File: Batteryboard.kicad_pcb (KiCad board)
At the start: 4 copper layers, 75.8 x 76.2 mm, 143 parts, among them IC1 FAN4010IL6X_F113, IC2 FAN4010IL6X_F113, IC3 FAN4010IL6X_F113, J1 Conn_01x02_Male, J2 Conn_01x03_Male, J4 Conn_01x02_Male, J5 SC_19-20, Q1 SI7617DN-T1-GE3, Q2 SI7617DN-T1-GE3, Q3 SI7617DN-T1-GE3, Q4 SIS412DN-T1-GE3, Q5 SIS412DN-T1-GE3, Q6 SIS412DN-T1-GE3, Q7 SI7617DN-T1-GE3, Q8 SIS412DN-T1-GE3, U1 BQ24617RGET, U2 TPS65279DAPR, U3 BQ29200DRBT, U4 PIC18F25K50-I_SO, U5 MCP2515-xSO, U6 SN65HVD1050D

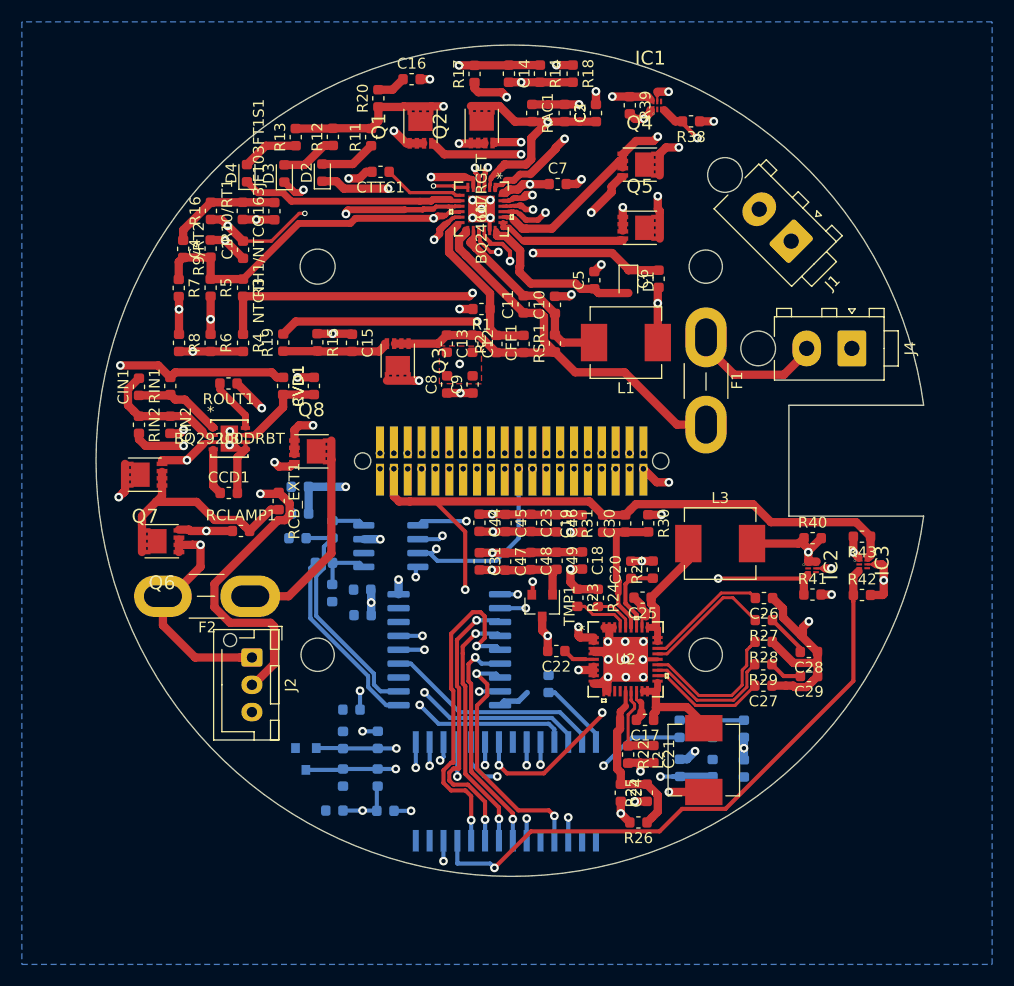
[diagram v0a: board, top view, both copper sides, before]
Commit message: complete overhaul of board, trying to make it a bit better
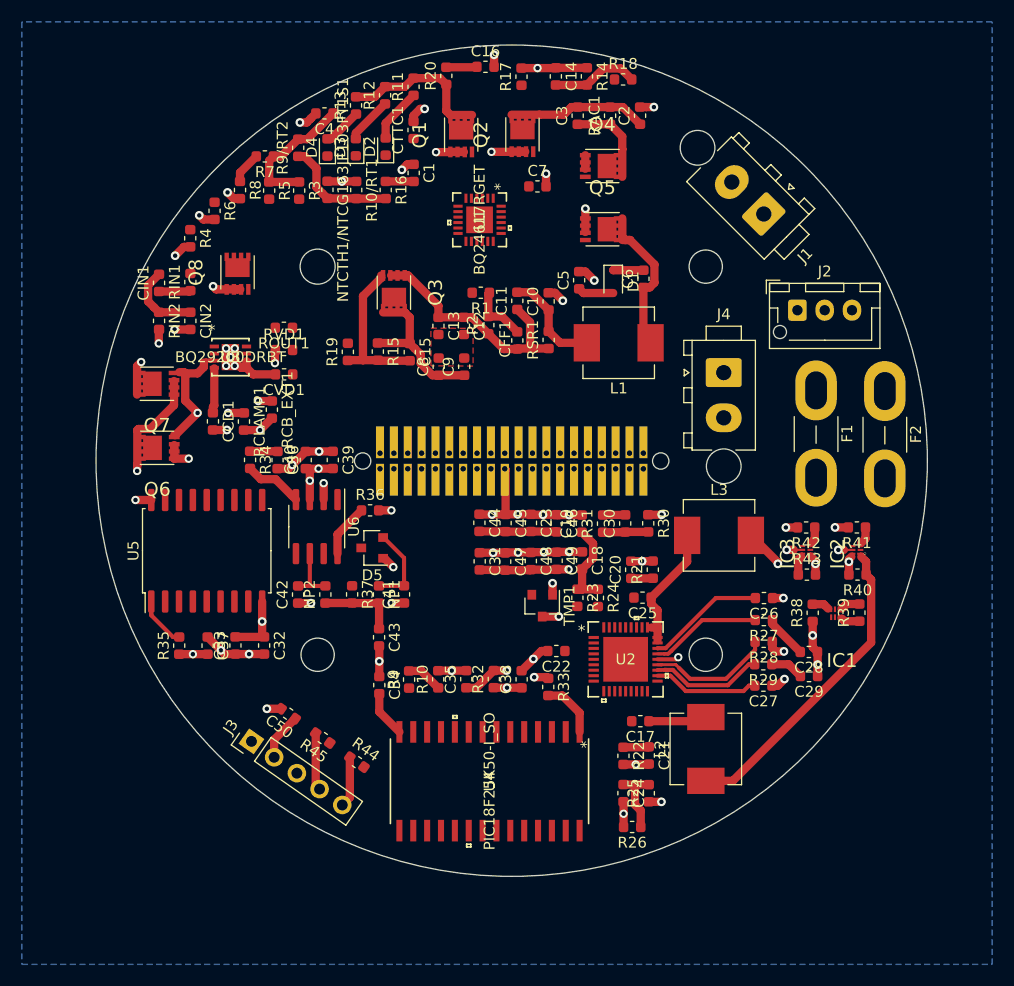
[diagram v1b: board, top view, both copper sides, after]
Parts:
- added C50: C, Capacitor_SMD:C_0603_1608Metric, F.Cu at (214.9, 86.2)
- added J3: Conn_01x05_Male, Connector_PinHeader_2.54mm:PinHeader_1x05_P2.54mm_Vertical, F.Cu at (211.5, 88.8)
- added R44: R_US, Resistor_SMD:R_0603_1608Metric, F.Cu at (221.2, 90.7)
- added R45: R_US, Resistor_SMD:R_0603_1608Metric, F.Cu at (218.1, 88.5)
- C32, C33, C34, C35, C36, C37, C38, C39, C40, C41, C42, C43, D5, NP1, NP2, R10, R32, R33, R34, R35, R36, R37, R9, U4, U5, U6: moved to F.Cu
- moved F2 61.1 mm to (269.6, 56.7), turned to 270 degrees
- moved J2 59.2 mm to (261.6, 49.3), turned to 0 degrees
- moved R39 51.0 mm to (267.2, 77.0), turned to 90 degrees
- moved IC1 49.3 mm to (265.0, 77.0), turned to 180 degrees
- moved R38 46.4 mm to (263.0, 77.0), turned to 90 degrees
- moved R10 26.4 mm to (228.7, 83.1)
- moved R9 26.1 mm to (226.0, 83.1), turned to 90 degrees
- moved U5 24.0 mm to (207.4, 71.3), turned to 90 degrees
- moved R32 23.4 mm to (233.7, 83.1)
- moved C35 23.0 mm to (231.2, 83.1), turned to 90 degrees
- moved C38 21.9 mm to (236.3, 83.1), turned to 90 degrees
- moved D5 20.3 mm to (222.6, 71.1), turned to 180 degrees
- moved R37 20.1 mm to (220.8, 75.3), turned to 270 degrees
- moved R36 18.3 mm to (222.4, 67.6), turned to 0 degrees
- moved Q8 17.7 mm to (210.3, 45.8), turned to 90 degrees
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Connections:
- C15 pad 1: 5V0 -> Q4D
- C23 pad 2: 5V0 -> Net-(C23-Pad2)
- C3 pad 1: 5V0 -> Q4D
- C31 pad 2: 5V0 -> Net-(C31-Pad2)
- C44 pad 2: 5V0 -> Net-(C23-Pad2)
- C45 pad 2: 5V0 -> Net-(C23-Pad2)
- C46 pad 2: 5V0 -> Net-(C23-Pad2)
- C47 pad 2: 5V0 -> Net-(C31-Pad2)
- C48 pad 2: 5V0 -> Net-(C31-Pad2)
- C49 pad 2: 5V0 -> Net-(C31-Pad2)
- C8 pad 1: 5V0 -> Q4D
- C9 pad 1: 5V0 -> Q4D
- IC1 pad 1: 5V0 -> Q4D
- IC2 pad 1: 5V0 -> Net-(C23-Pad2)
- IC3 pad 1: 5V0 -> Net-(C31-Pad2)
- L2 pad 1: 5V0 -> Net-(C23-Pad2)
- L3 pad 2: 5V0 -> Net-(C31-Pad2)
- Q3 pad 5: 5V0 -> Q4D
- Q3 pad 6: 5V0 -> Q4D
- Q3 pad 7: 5V0 -> Q4D
- Q3 pad 8: 5V0 -> Q4D
- Q4 pad 5: 5V0 -> Q4D
- Q4 pad 6: 5V0 -> Q4D
- Q4 pad 7: 5V0 -> Q4D
- Q4 pad 8: 5V0 -> Q4D
- R15 pad 1: 5V0 -> Q4D
- R39 pad 2: 5V0 -> Q4D
- R40 pad 1: 5V0 -> Net-(C23-Pad2)
- R43 pad 2: 5V0 -> Net-(C31-Pad2)
- RAC1 pad 1: 5V0 -> Q4D
- U1 pad 1: 5V0 -> Q4D
- U4 pad 27: Net-(U4-Pad27) -> PGC
- U4 pad 28: Net-(U4-Pad28) -> PGD
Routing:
- net TS: track 115.4 -> 2.56 mm, vias 4 -> 0
- net VBATCURRENT: track 96.1 -> 2.43 mm, vias 2 -> 0
- net VBAT: track 98.5 -> 10.3 mm, vias 6 -> 0
- net 3V3: track 92.6 -> 8.80 mm, vias 6 -> 0
- net 5V0: track 94.7 -> 19.5 mm, vias 25 -> 7
- net 3V3CURRENT: track 56.2 -> 2.45 mm, vias 1 -> 0
- net PGND2: track 157.1 -> 112.7 mm, vias 45 -> 59
- net Net-(J1-Pad1): track 57.1 -> 14.1 mm, vias 1 -> 0
- net 5VCURRENT: track 44.0 -> 2.44 mm, vias 3 -> 0
- net CAN_L: track 46.2 -> 5.47 mm, vias 3 -> 0
- net Q6S: track 56.9 -> 17.4 mm
- net CAN_H: track 46.1 -> 7.55 mm, vias 3 -> 0
- net Net-(C31-Pad2): track 0.00 -> 37.5 mm, vias 0 -> 3
- net Net-(C23-Pad2): track 0.00 -> 36.7 mm
- net ISET2: track 36.3 -> 0.00 mm, vias 2 -> 0
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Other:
- board size 75.8 x 76.2 mm -> 76.2 x 76.2 mm
